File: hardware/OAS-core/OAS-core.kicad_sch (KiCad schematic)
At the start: 29 parts, among them J1 Micro_SD_Card, J2 PROG, J3 MSC, J4 XT30PW-M, Q1 PMOS, Q2 PMOS, U1 ESP32-WROOM-32, U2 TPS2116DRL, U3 TPS2116DRL, U4 TPS26600, U5 TPS563202DRLR, U6 TPS5430DDA, U7 LM66100DCK

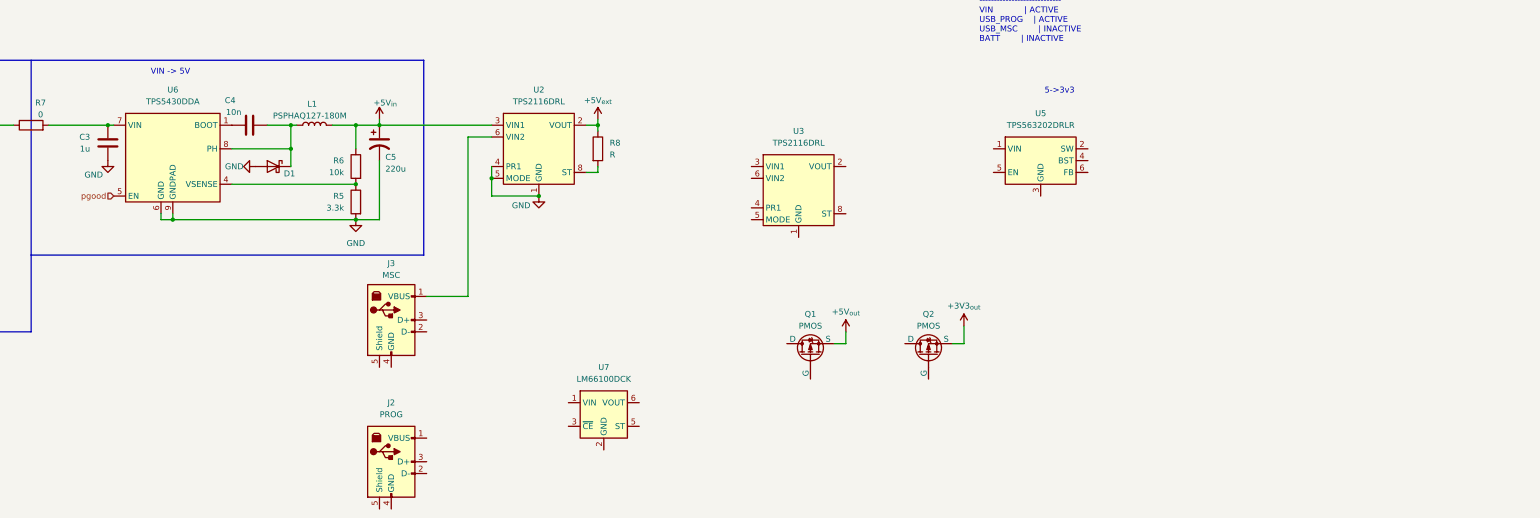
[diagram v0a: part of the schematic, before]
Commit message: PSU Mux
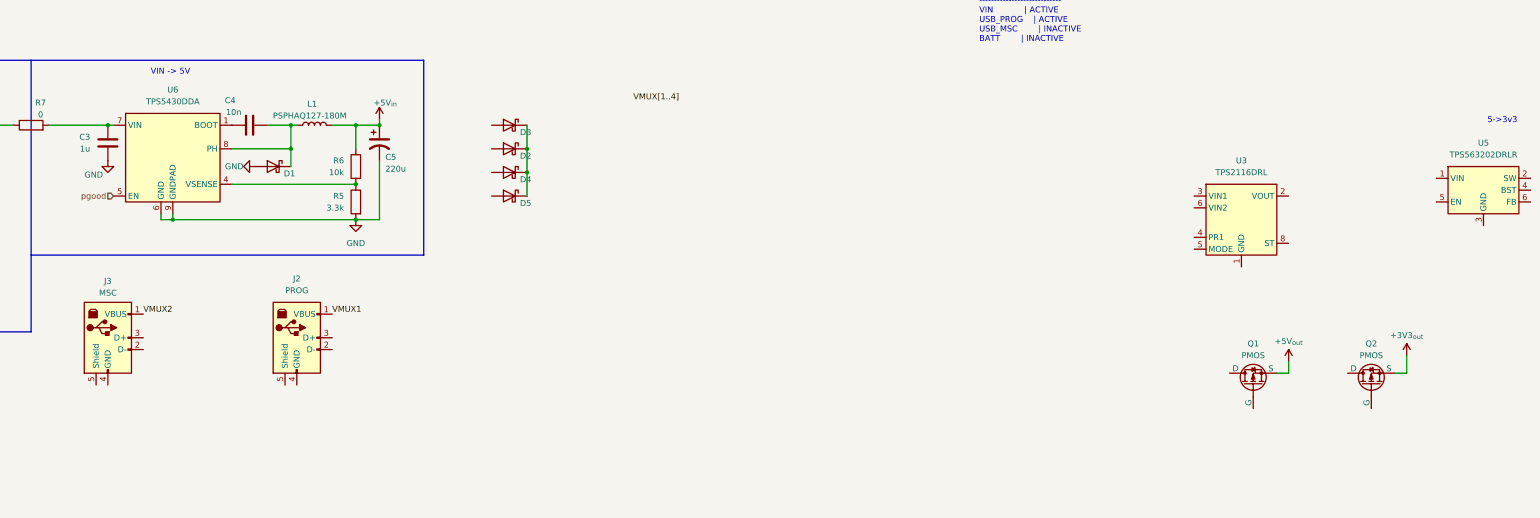
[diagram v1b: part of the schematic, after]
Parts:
- removed R8: R, symbol Device:R
- removed U2: TPS2116DRL, Package_TO_SOT_SMD:SOT-583-8, symbol Power_Management:TPS2116DRL
- removed U7: LM66100DCK, Package_TO_SOT_SMD:SOT-363_SC-70-6, symbol Power_Management:LM66100DCK
- added D2, D3, D4, D5: SS54, Diode_SMD:D_SMA, symbol Device:D_Schottky
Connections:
- net VMUX2: now reaches J3.1 (VBUS)
- net VMUX1: now reaches J2.1 (VBUS)
- new net: D2.1 (K), D3.1 (K), D4.1 (K), D5.1 (K)
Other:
- moved on the sheet: J2, J3, Q1, Q2, U3, U5
